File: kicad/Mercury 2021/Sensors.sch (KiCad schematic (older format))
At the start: 17 parts, among them J16 Sensors_Extra, J17 Arduino_Extra_Power, J18 Arduino_Extra_Comm, J19 Arduino_Extra_Digital, J20 Arduino_Extra_Analog, J21 MP_Extra_Analog, J39 USB_A, U10 TCA9548APWR, U2 Adafruit_VL53L0X, U3 Adafruit_VL53L0X, U4 Adafruit_VL53L0X, U5 Adafruit_VL53L0X, U6 Adafruit_VL53L0X, U7 Adafruit_VL53L0X, U8 Adafruit_VL53L0X, U9 Adafruit_VL53L0X

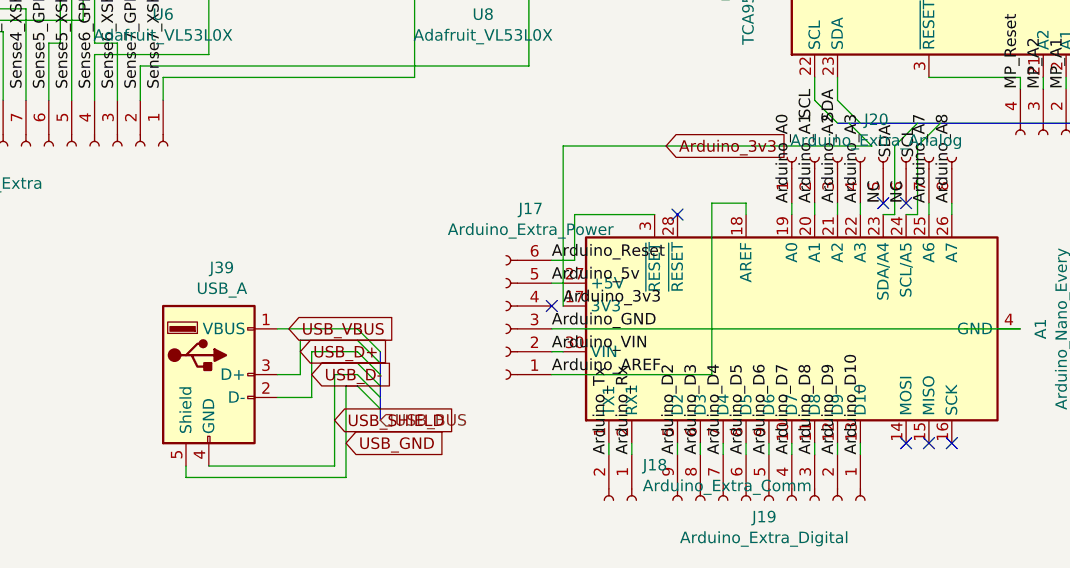
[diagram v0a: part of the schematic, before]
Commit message: New New board
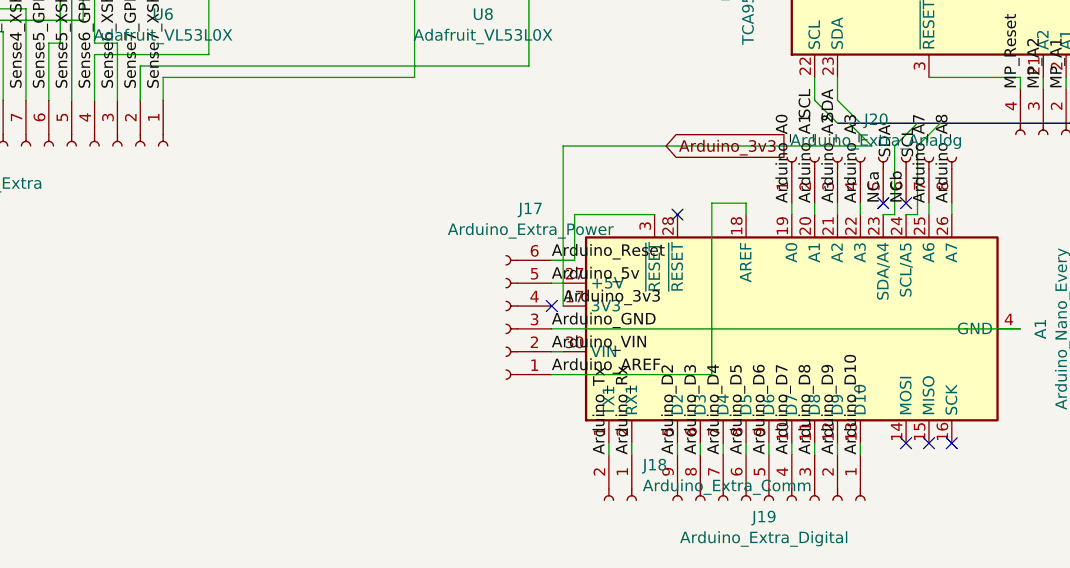
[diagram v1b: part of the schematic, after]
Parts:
- removed J39: USB_A, Connector_USB:USB_A_Molex_105057_Vertical, symbol Connector:USB_A
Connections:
- net NC renamed NCa
- net NCa: no longer J20.6 (Pin_6)
- new net NCb: J20.6 (Pin_6)
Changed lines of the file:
@@
 Arduino_A3
 Text Label 7400 3450 1    50   ~ 0
-NC
-Text Label 7500 3450 1    50   ~ 0
-NC
+NCa
 Text Label 7700 3450 1    50   ~ 0
 Arduino_A8
@@
 Text GLabel 6450 3200 2    50   Input ~ 0
 Arduino_3v3
-Text HLabel 5200 4400 2    50   Input ~ 0
-USB_BUS
-$Comp
-L Connector:USB_A J39
-U 1 1 612C23CD
-P 4450 4200
-F 0 "J39" H 4507 4667 50  0000 C CNN
-F 1 "USB_A" H 4507 4576 50  0000 C CNN
-F 2 "Connector_USB:USB_A_Molex_105057_Vertical" H 4600 4150 50  0001 C CNN
-F 3 " ~" H 4600 4150 50  0001 C CNN
-	1    4450 4200
-	1    0    0    -1
-$EndComp
-Wire Wire Line
-	4750 4200 4850 4200
-Wire Wire Line
-	4850 4200 4850 4050
-Wire Wire Line
-	4750 4300 4900 4300
-Wire Wire Line
-	4900 4300 4900 4100
-Wire Wire Line
-	4450 4600 5000 4600
-Wire Wire Line
-	5000 4600 5000 4200
-Wire Wire Line
-	4350 4600 4350 4650
-Wire Wire Line
-	4350 4650 5050 4650
-Wire Wire Line
-	5050 4250 5100 4250
-Wire Wire Line
-	5000 4200 5100 4200
-Wire Wire Line
-	4950 4150 5100 4150
-Wire Wire Line
-	4900 4100 5100 4100
-Wire Wire Line
-	4850 4050 5100 4050
-Entry Wire Line
-	5100 4000 5200 4100
-Entry Wire Line
-	5100 4050 5200 4150
-Entry Wire Line
-	5100 4100 5200 4200
-Entry Wire Line
-	5100 4150 5200 4250
-Entry Wire Line
-	5100 4200 5200 4300
-Entry Wire Line
-	5100 4250 5200 4350
-Text GLabel 4800 4000 2    50   Input ~ 0
-USB_VBUS
-Text GLabel 4850 4100 2    50   Input ~ 0
-USB_D+
-Text GLabel 4900 4200 2    50   Input ~ 0
-USB_D-
-Text GLabel 5000 4400 2    50   Input ~ 0
-USB_SHIELD
-Text GLabel 5050 4500 2    50   Input ~ 0
-USB_GND
 Wire Wire Line
 	1900 2850 2850 2850
@@
 Wire Wire Line
 	5950 4000 8000 4000
-Wire Wire Line
-	5100 4000 4750 4000
-Wire Wire Line
-	5050 4250 5050 4650
-Wire Bus Line
-	5200 4100 5200 4400
 Wire Bus Line
 	9000 3000 9550 3000
 Wire Bus Line
+	7200 3100 9000 3100
+Wire Bus Line
 	9650 1850 9650 2600
 Wire Bus Line
 	9000 1850 9000 3000
 Wire Bus Line
-	7200 3100 9000 3100
+	6700 1850 9000 1850
 Wire Bus Line
 	700  1650 6700 1650
-Wire Bus Line
-	6700 1850 9000 1850
+Text Label 7500 3450 1    50   ~ 0
+NCb
 $EndSCHEMATC
